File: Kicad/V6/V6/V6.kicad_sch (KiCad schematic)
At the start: 17 parts, among them J1 Conn_01x05_Pin, J39 Conn_01x02_Pin, U1 WPME-FDSM_SIP-3, U3 MCP23017-E/SO, U4 ISOM8600DFGR, U5 TLV75533PDYDR, U7 INA237AIDGSR

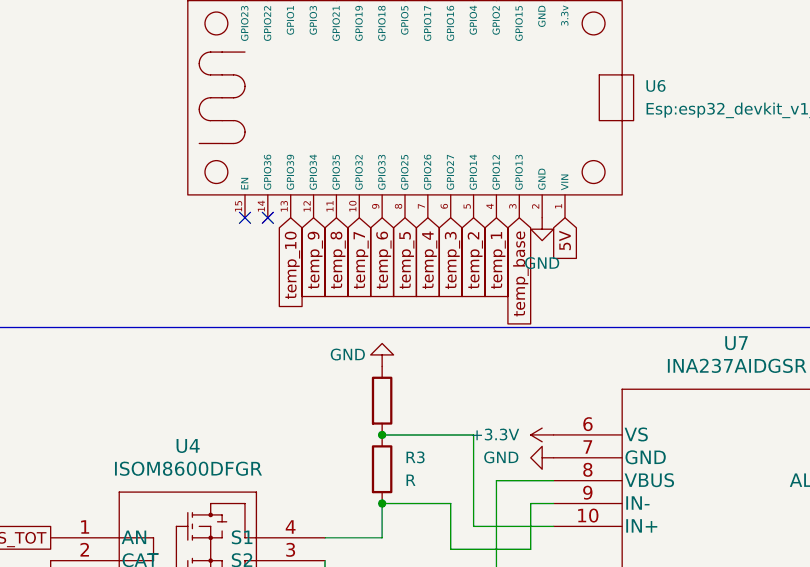
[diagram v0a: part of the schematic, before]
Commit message: Pojet batterie fonctionne, plus création du readme
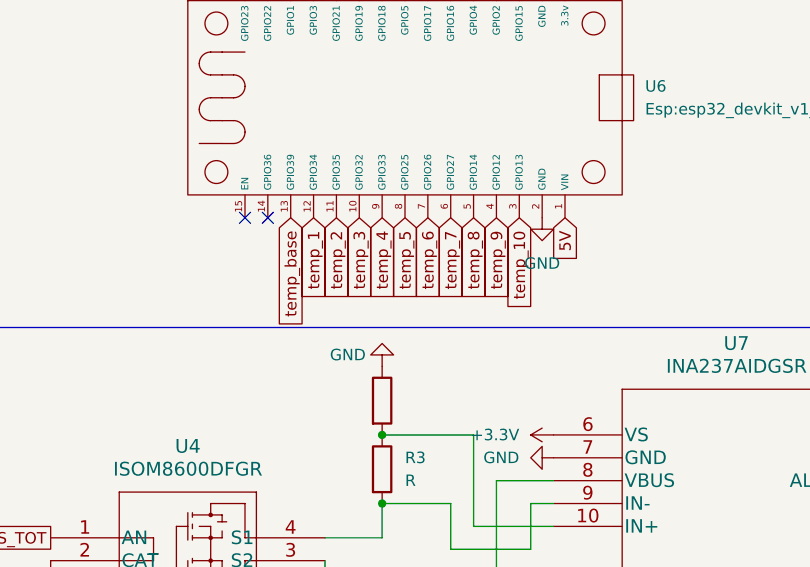
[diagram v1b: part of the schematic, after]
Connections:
- net temp_1: now also U6.12 (GPIO34); no longer U6.4 (GPIO12)
- net temp_10: now also U6.3 (GPIO13); no longer U6.13 (GPIO39)
- net temp_2: now also U6.11 (GPIO35); no longer U6.5 (GPIO14)
- net temp_3: now also U6.10 (GPIO32); no longer U6.6 (GPIO27)
- net temp_4: now also U6.9 (GPIO33); no longer U6.7 (GPIO26)
- net temp_6: now also U6.7 (GPIO26); no longer U6.9 (GPIO33)
- net temp_7: now also U6.6 (GPIO27); no longer U6.10 (GPIO32)
- net temp_8: now also U6.5 (GPIO14); no longer U6.11 (GPIO35)
- net temp_9: now also U6.4 (GPIO12); no longer U6.12 (GPIO34)
- net temp_base: now also U6.13 (GPIO39); no longer U6.3 (GPIO13)
